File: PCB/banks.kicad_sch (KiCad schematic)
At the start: 50 parts, among them U1 XC7A50T-FGG484, Y3 100MHz

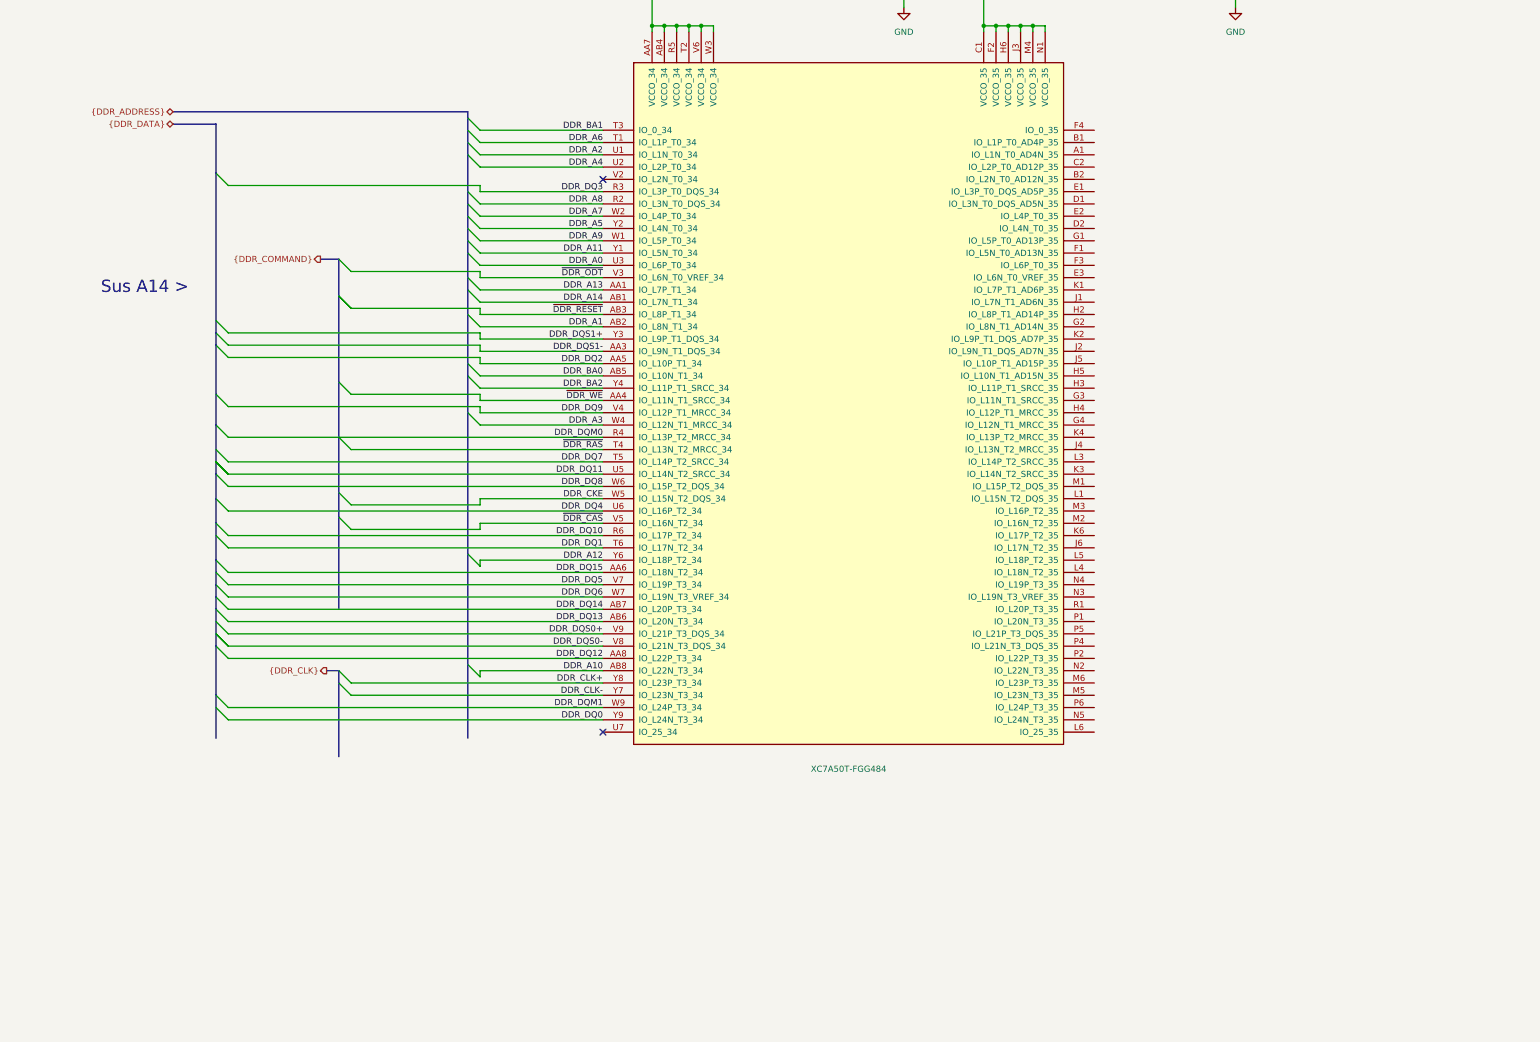
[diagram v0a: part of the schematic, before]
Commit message: 5th time routing is the charm EHH :D
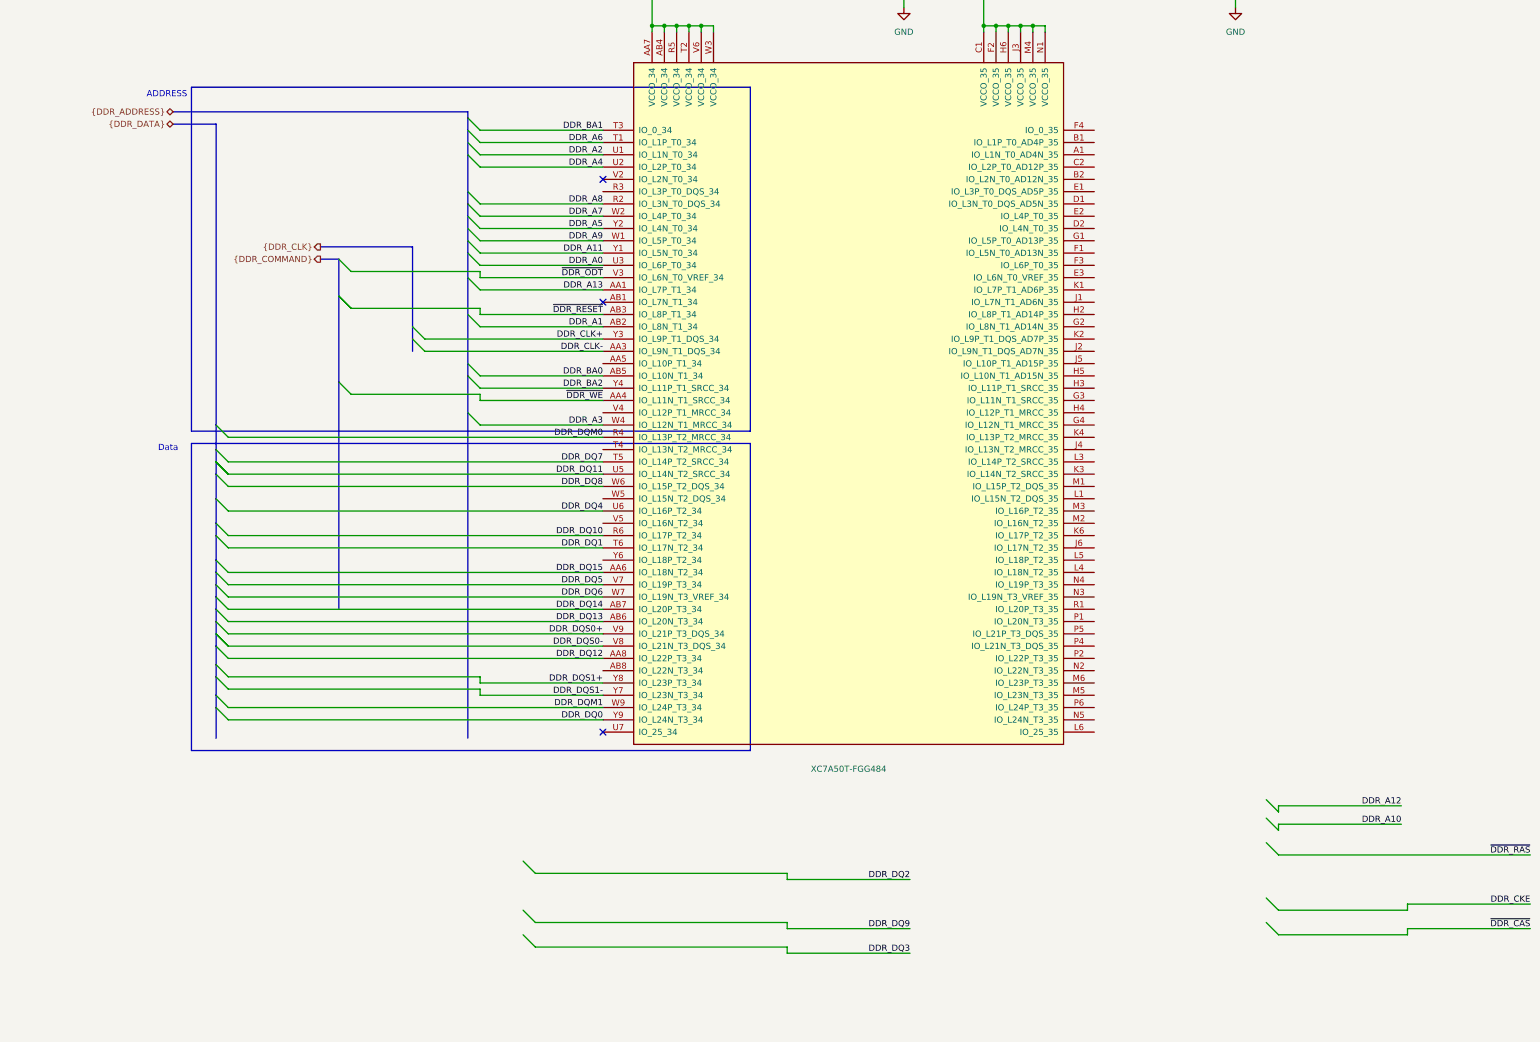
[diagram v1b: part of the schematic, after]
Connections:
- net DDR_A10: no longer U1.AB8 (IO_L22N_T3_34)
- net DDR_A12: no longer U1.Y6 (IO_L18P_T2_34)
- net DDR_CKE: no longer U1.W5 (IO_L15N_T2_DQS_34)
- net DDR_CLK+: now also U1.Y3 (IO_L9P_T1_DQS_34); no longer U1.Y8 (IO_L23P_T3_34)
- net DDR_CLK-: now also U1.AA3 (IO_L9N_T1_DQS_34); no longer U1.Y7 (IO_L23N_T3_34)
- net DDR_DQ2: no longer U1.AA5 (IO_L10P_T1_34)
- net DDR_DQ3: no longer U1.R3 (IO_L3P_T0_DQS_34)
- net DDR_DQ9: no longer U1.V4 (IO_L12P_T1_MRCC_34)
- net DDR_DQS1+: now also U1.Y8 (IO_L23P_T3_34); no longer U1.Y3 (IO_L9P_T1_DQS_34)
- net DDR_DQS1-: now also U1.Y7 (IO_L23N_T3_34); no longer U1.AA3 (IO_L9N_T1_DQS_34)
- net ~{DDR_CAS}: no longer U1.V5 (IO_L16N_T2_34)
- net ~{DDR_RAS}: no longer U1.T4 (IO_L13N_T2_MRCC_34)
- net DDR_A14: no longer names the net of U1.AB1 (IO_L7N_T1_34)
- no-connect marks 12 -> 13
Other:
- note added: "ADDRESS"
- note added: "Data"
- note removed: "Sus A14 >"
